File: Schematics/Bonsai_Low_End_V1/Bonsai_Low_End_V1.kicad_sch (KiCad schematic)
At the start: 23 parts, among them J1 Bat_Connector, U1 MOUDLE-SEEEDUINO-XIAO-ESP32C3, U2 MAX30101EFD, U3 1.8V, U5 DRV2605LDGS

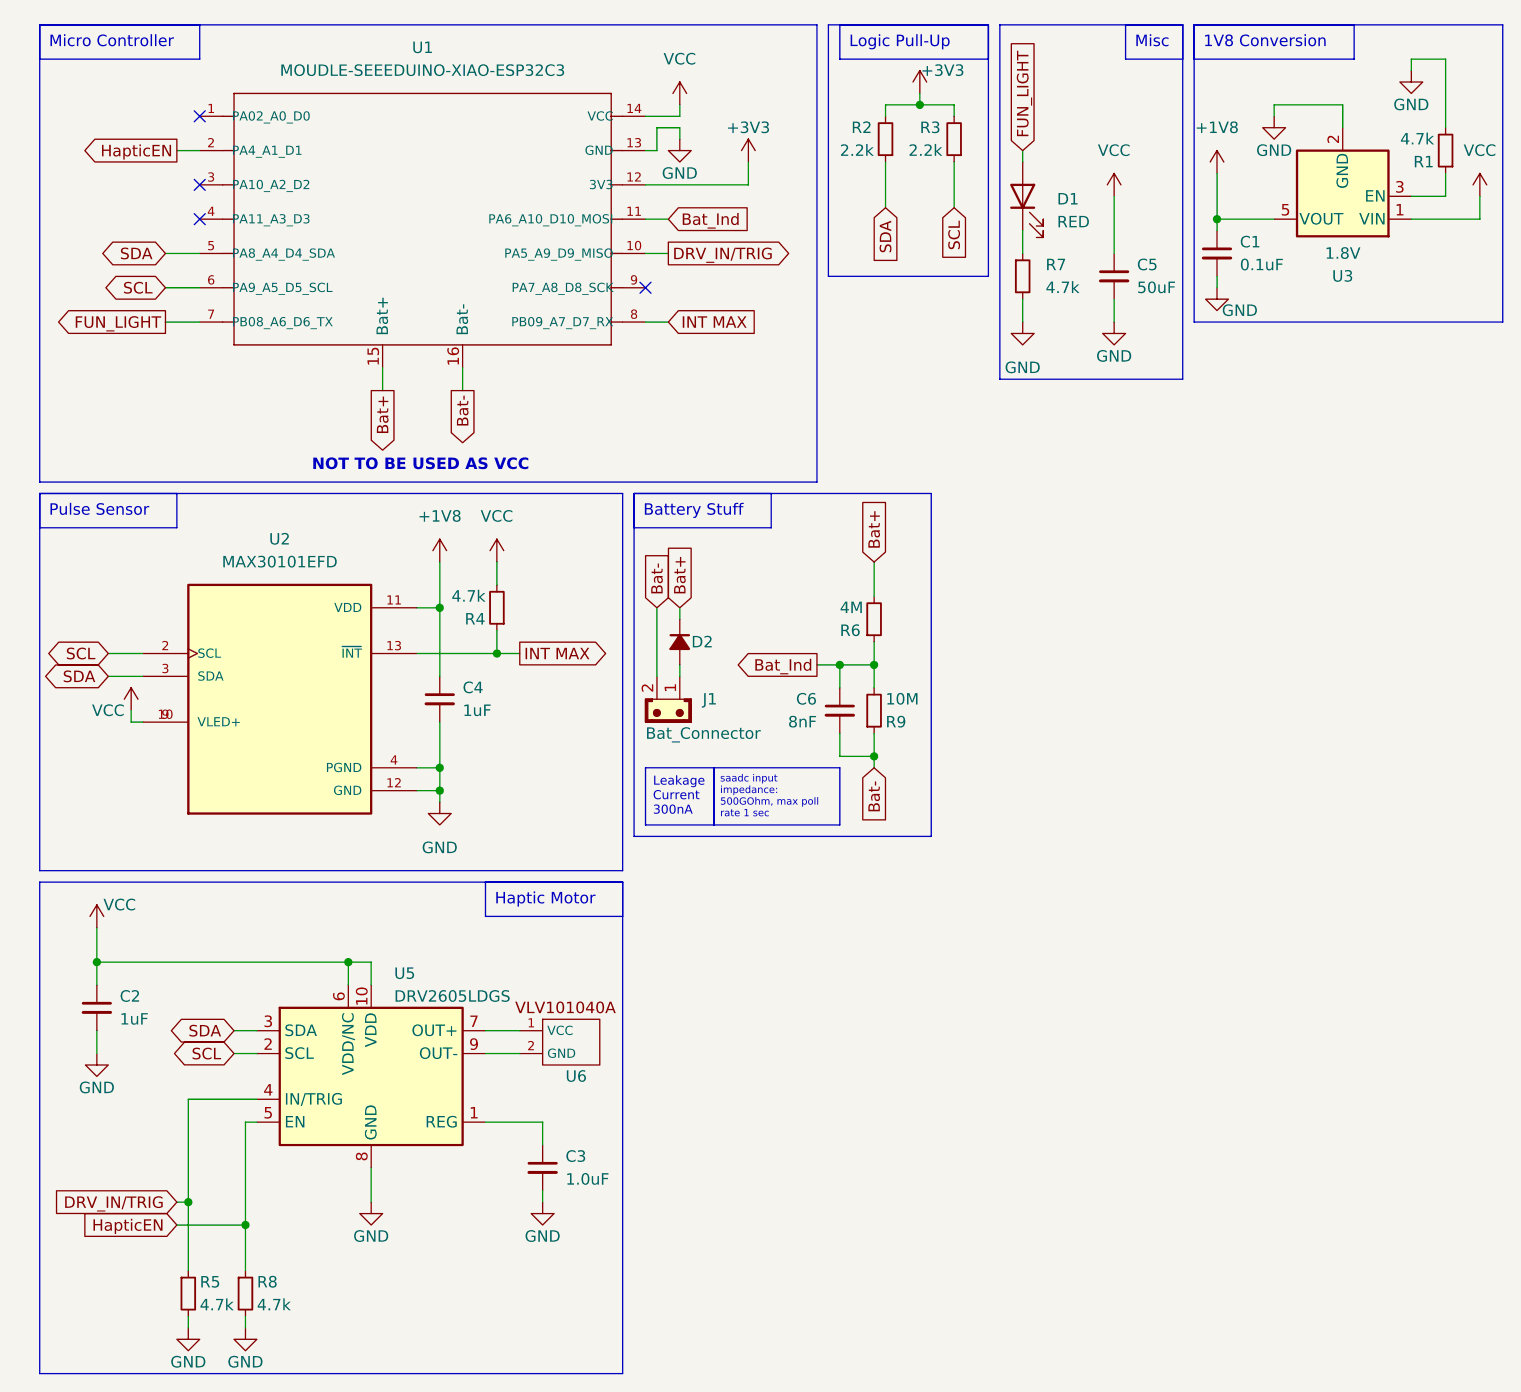
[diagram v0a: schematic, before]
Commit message: finished pcb
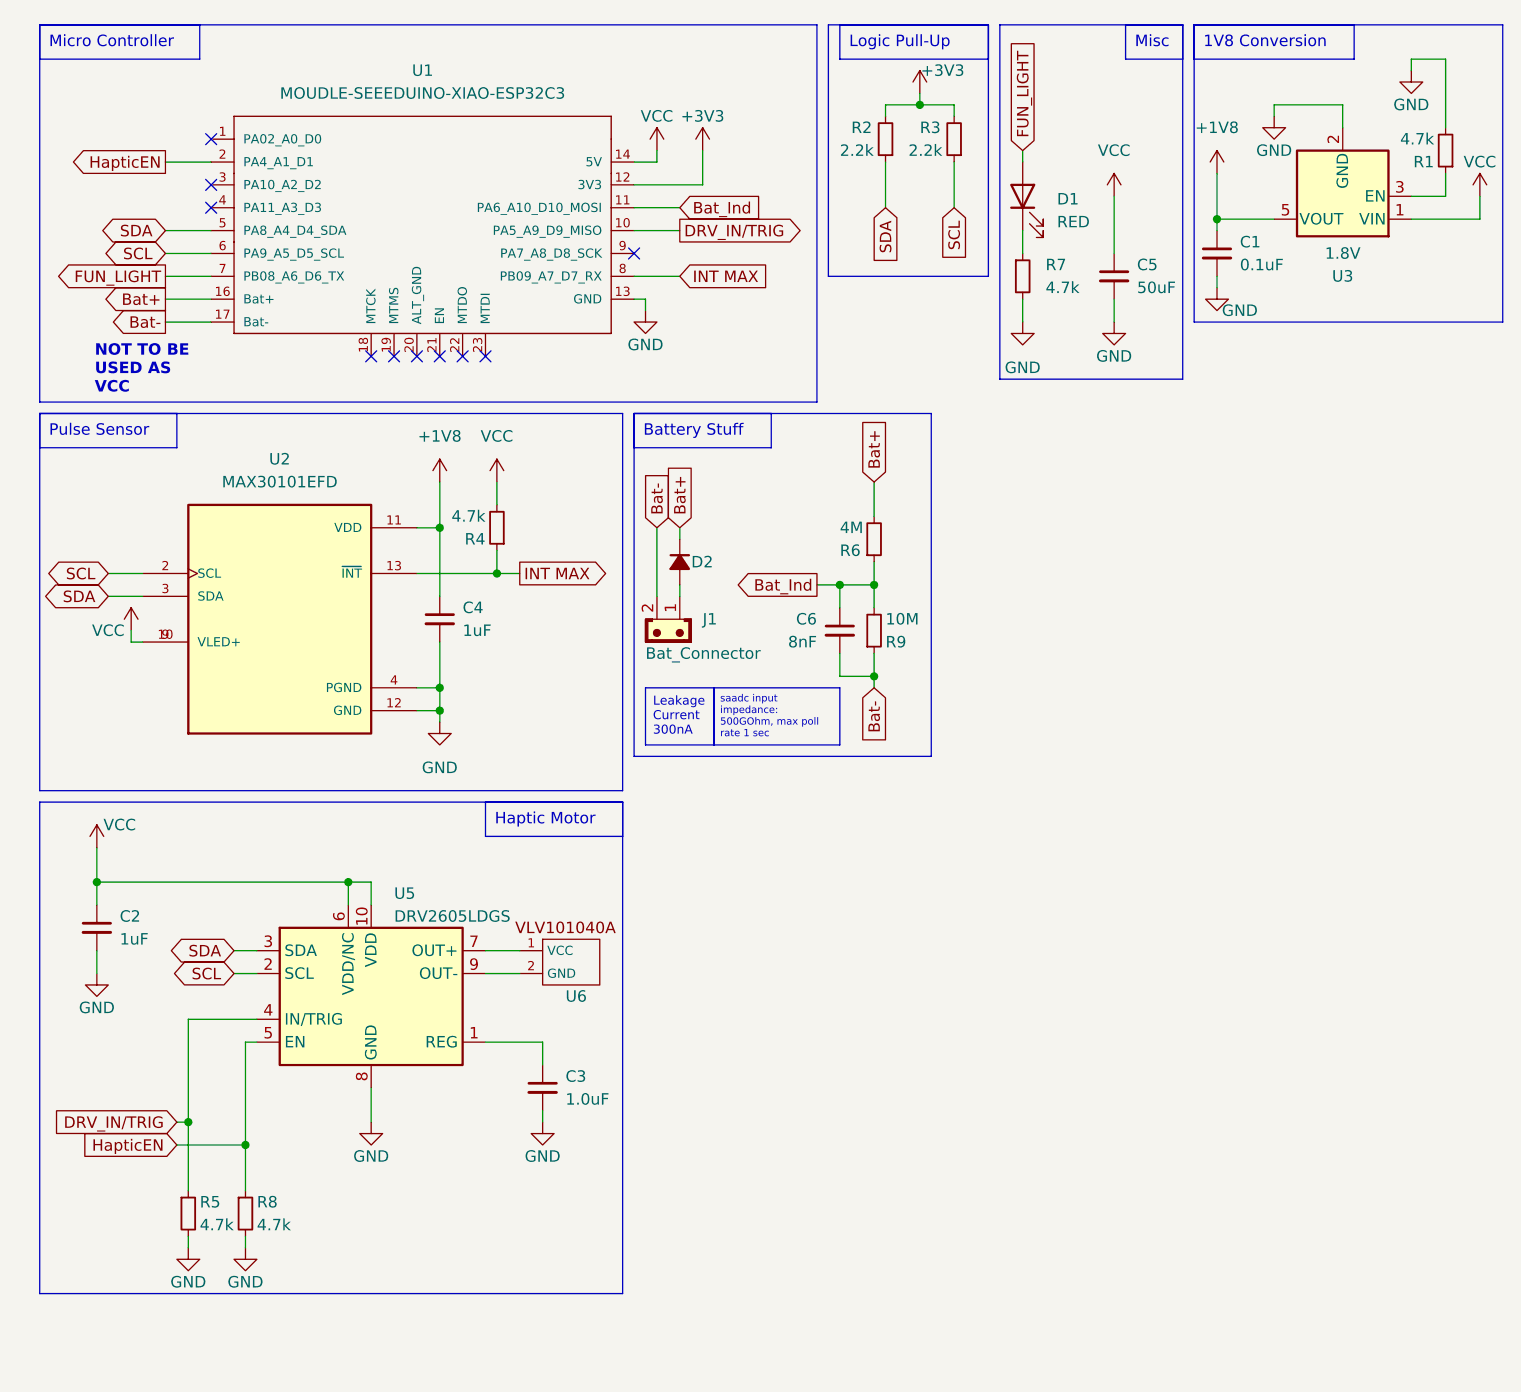
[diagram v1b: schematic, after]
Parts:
- U1: footprint xiao ESP32C3_PCB:MOUDLE14P-SMD-2.54-21X17.8MM -> xiao ESP32C3_PCB:xiap esp32c3_PCB_ ADDED BATTERY PADS
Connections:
- net Bat+: now also U1.16 (Bat+); no longer U1.15 (Bat+)
- net Bat-: now also U1.17 (Bat-); no longer U1.16 (Bat-)
- no-connect marks 4 -> 10
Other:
- moved on the sheet: C2, C3, C4, C6, D2, J1, R4, R5, R6, R8, R9, U2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
